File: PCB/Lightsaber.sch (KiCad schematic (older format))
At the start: 10 parts, among them Q1 SS8050, Q2 SS8050, Q3 SS8050, SW1 SW_Push

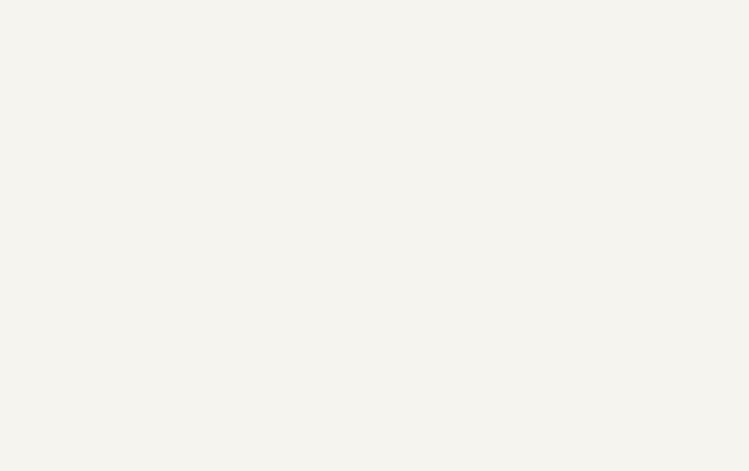
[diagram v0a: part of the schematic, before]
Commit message: update
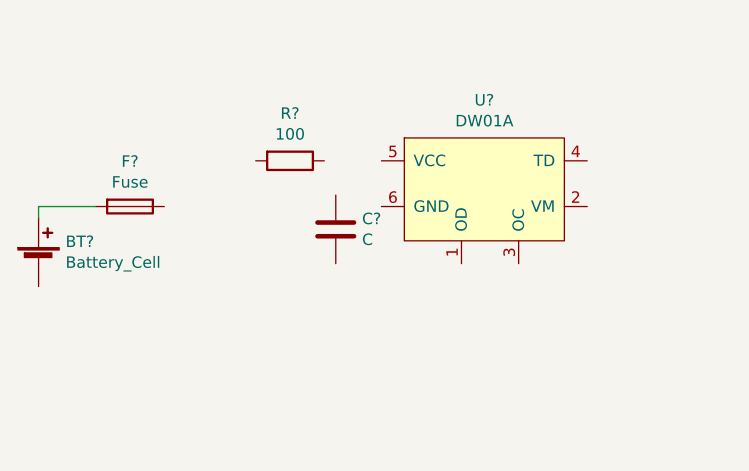
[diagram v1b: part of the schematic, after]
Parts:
- added BT?: Battery_Cell, symbol Device:Battery_Cell
- added C?: C, symbol Device:C
- added F?: Fuse, symbol Device:Fuse
- added R?: 100, symbol Device:R
- added U?: DW01A, symbol Lightsaber_custom:DW01A
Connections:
- new net: BT?.1 (+), F?.2
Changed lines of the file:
@@
 Wire Wire Line
 	9800 3250 9800 3400
+$Comp
+L Device:Battery_Cell BT?
+U 1 1 631E3320
+P 800 1800
+F 0 "BT?" H 918 1896 50  0000 L CNN
+F 1 "Battery_Cell" H 918 1805 50  0000 L CNN
+F 2 "" V 800 1860 50  0001 C CNN
+F 3 "~" V 800 1860 50  0001 C CNN
+	1    800  1800
+	1    0    0    -1
+$EndComp
+$Comp
+L Device:Fuse F?
+U 1 1 631E4D50
+P 1200 1550
+F 0 "F?" V 1003 1550 50  0000 C CNN
+F 1 "Fuse" V 1094 1550 50  0000 C CNN
+F 2 "" V 1130 1550 50  0001 C CNN
+F 3 "~" H 1200 1550 50  0001 C CNN
+	1    1200 1550
+	0    1    1    0
+$EndComp
+Wire Wire Line
+	800  1600 800  1550
+Wire Wire Line
+	800  1550 1050 1550
+$Comp
+L Lightsaber_custom:DW01A U?
+U 1 1 631E6E9D
+P 2800 1150
+F 0 "U?" H 2750 1215 50  0000 C CNN
+F 1 "DW01A" H 2750 1124 50  0000 C CNN
+F 2 "" H 2750 1200 50  0001 C CNN
+F 3 "" H 2750 1200 50  0001 C CNN
+	1    2800 1150
+	1    0    0    -1
+$EndComp
+$Comp
+L Device:R R?
+U 1 1 631E7B9E
+P 1900 1350
+F 0 "R?" V 1693 1350 50  0000 C CNN
+F 1 "100" V 1784 1350 50  0000 C CNN
+F 2 "" V 1830 1350 50  0001 C CNN
+F 3 "~" H 1900 1350 50  0001 C CNN
+	1    1900 1350
+	0    1    1    0
+$EndComp
+$Comp
+L Device:C C?
+U 1 1 631E8406
+P 2100 1650
+F 0 "C?" H 2215 1696 50  0000 L CNN
+F 1 "C" H 2215 1605 50  0000 L CNN
+F 2 "" H 2138 1500 50  0001 C CNN
+F 3 "~" H 2100 1650 50  0001 C CNN
+	1    2100 1650
+	1    0    0    -1
+$EndComp
 $EndSCHEMATC
